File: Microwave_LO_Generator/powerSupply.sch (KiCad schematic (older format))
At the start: 26 parts, among them IC1 ADP150AUJZ-3.3-R7, U2 LM317L_SO8, U3 LM317L_SO8

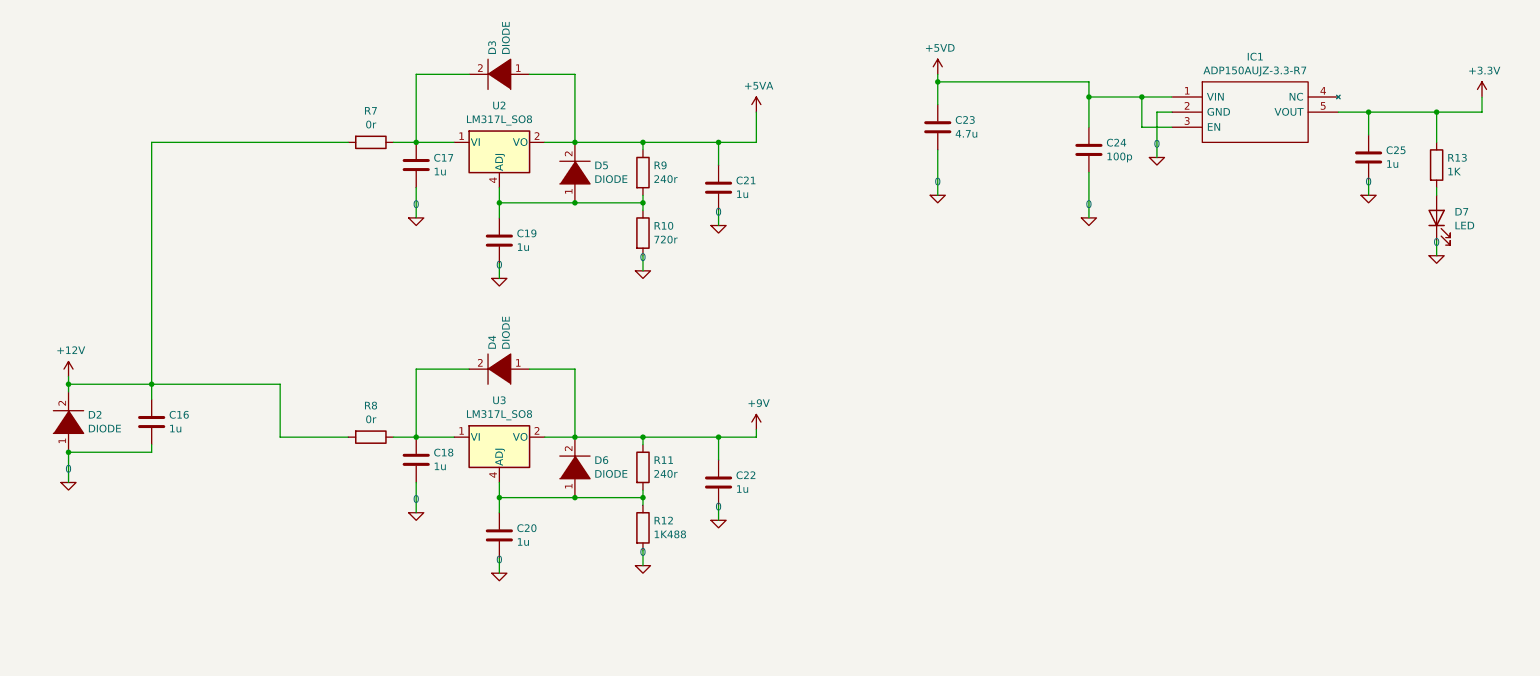
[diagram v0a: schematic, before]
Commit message: Power Supply update
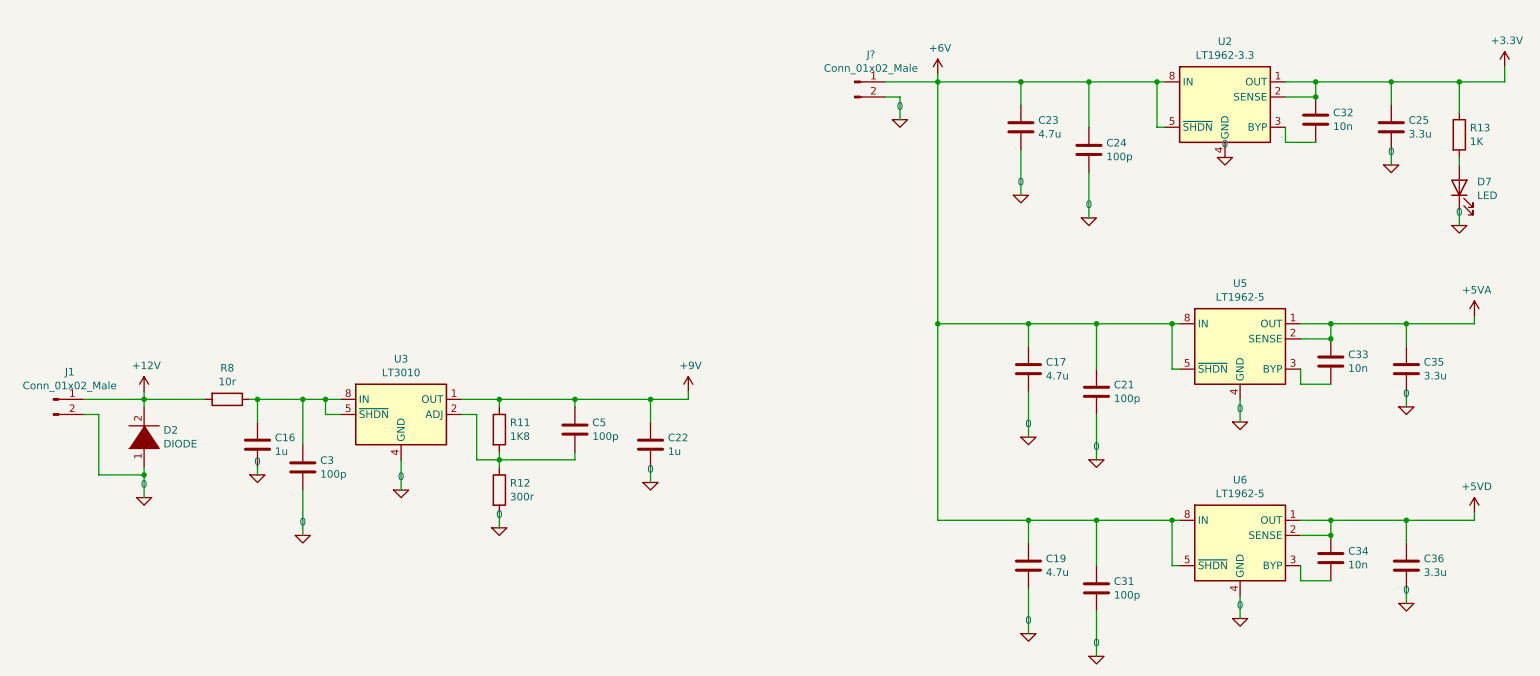
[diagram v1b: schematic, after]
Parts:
- removed C18, C20: 1u, Capacitor_SMD:C_0402_1005Metric_Pad0.74x0.62mm_HandSolder, symbol Device:C
- removed D3, D4, D5, D6: DIODE, Diode_SMD:D_MELF, symbol pspice:DIODE
- removed IC1: ADP150AUJZ-3.3-R7, SamacSys_Parts:SOT95P280X100-5N, symbol SamacSys_Parts:ADP150AUJZ-3.3-R7
- removed R10: 720r, Resistor_SMD:R_0402_1005Metric_Pad0.72x0.64mm_HandSolder, symbol Device:R
- removed R7: 0r, Resistor_SMD:R_0402_1005Metric_Pad0.72x0.64mm_HandSolder, symbol Device:R
- removed R9: 240r, Resistor_SMD:R_0402_1005Metric_Pad0.72x0.64mm_HandSolder, symbol Device:R
- removed U2, U3: LM317L_SO8, Package_SO:SOIC-8_3.9x4.9mm_P1.27mm, symbol Regulator_Linear:LM317L_SO8
- added C3, C31, C5: 100p, Capacitor_SMD:C_0402_1005Metric_Pad0.74x0.62mm_HandSolder, symbol Device:C
- added C32, C33, C34: 10n, Capacitor_SMD:C_0402_1005Metric_Pad0.74x0.62mm_HandSolder, symbol Device:C
- added C35, C36: 3.3u, Capacitor_SMD:C_0402_1005Metric_Pad0.74x0.62mm_HandSolder, symbol Device:C
- added J1, J?: Conn_01x02_Male, Connector_PinHeader_2.54mm:PinHeader_1x02_P2.54mm_Vertical, symbol Connector:Conn_01x02_Male
- added U2: LT1962-3.3, Package_SO:MSOP-8_3x3mm_P0.65mm, symbol Regulator_Linear:LT1962-3.3
- added U3: LT3010, Package_SO:MSOP-8-1EP_3x3mm_P0.65mm_EP1.68x1.88mm, symbol Regulator_Linear:LT3010
- added U5, U6: LT1962-5, Package_SO:MSOP-8_3x3mm_P0.65mm, symbol Regulator_Linear:LT1962-5
- C17, C19: value 1u -> 4.7u
- C21: value 1u -> 100p
- C25: value 1u -> 3.3u
- R11: value 240r -> 1K8
- R12: value 1K488 -> 300r
- R8: value 0r -> 10r
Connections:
- net +12V: now also J1.1 (Pin_1); no longer C16.2
- net +3V3: now also C32.2, U2.1 (OUT), U2.2 (SENSE)
- net +5VA: now also C33.2, C35.2, U5.1 (OUT), U5.2 (SENSE); no longer C21.2
- net +5VD: now also C34.2, C36.2, U6.1 (OUT), U6.2 (SENSE); no longer C23.2, C24.2
- net +9V: now also C5.2, U3.1 (OUT)
- net 0: now also C3.1, C31.1, C35.1, C36.1, J1.2 (Pin_2), J?.2 (Pin_2), U2.4 (GND), U3.4 (GND), U3.9 (GND), U5.4 (GND), U6.4 (GND)
- net +6V: now reaches C17.2
- net +6V: now also C19.2, C21.2, C23.2, C24.2, C31.2, J?.1 (Pin_1), U2.5 (~SHDN), U2.8 (IN), U5.5 (~SHDN), U5.8 (IN), U6.5 (~SHDN), U6.8 (IN)
- net at R8.1: now also C16.2, C3.2, U3.5 (~SHDN), U3.8 (IN)
- net at R11.2, R12.1: now also C5.1, U3.2 (ADJ)
- new net: C32.1, U2.3 (BYP)
- new net: C33.1, U5.3 (BYP)
- new net: C34.1, U6.3 (BYP)
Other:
- moved on the sheet: C16, C22, C23, C25, D2, D7, R11, R12, R13, R8
